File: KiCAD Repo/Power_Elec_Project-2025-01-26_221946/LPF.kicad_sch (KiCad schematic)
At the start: 7 parts, among them U1 LM358

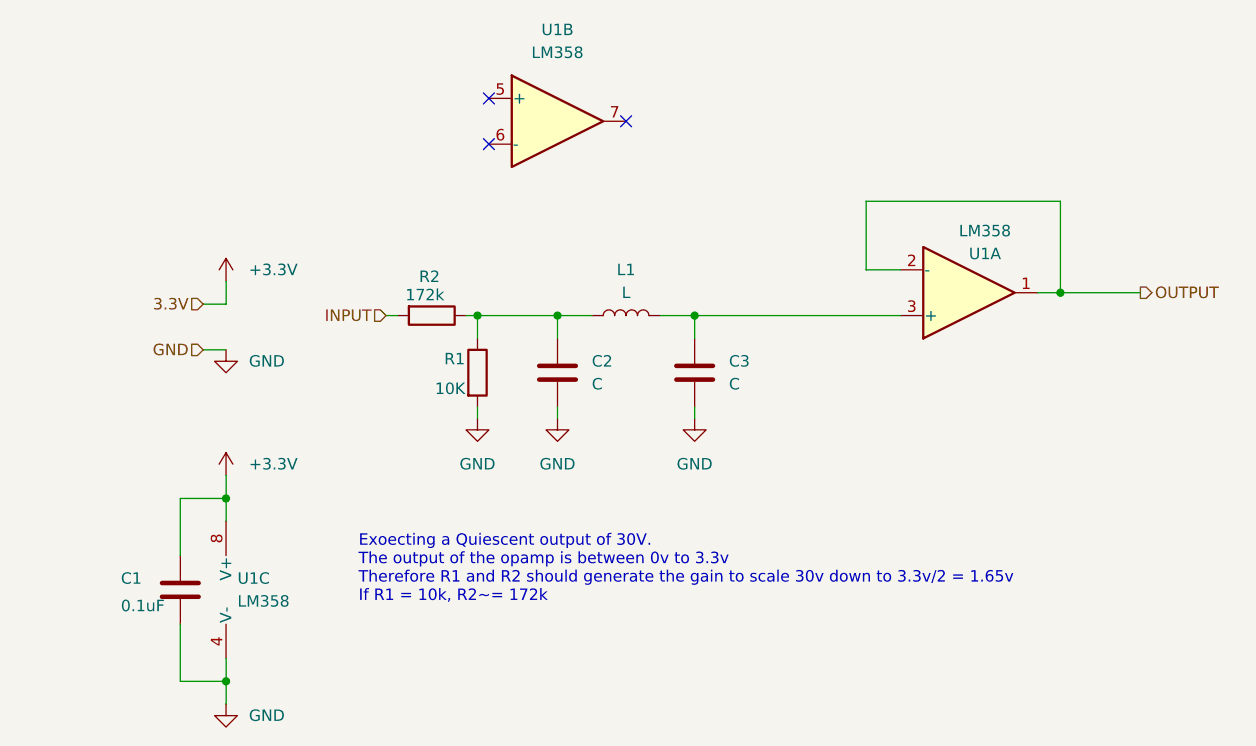
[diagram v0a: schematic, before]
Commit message: lpf design
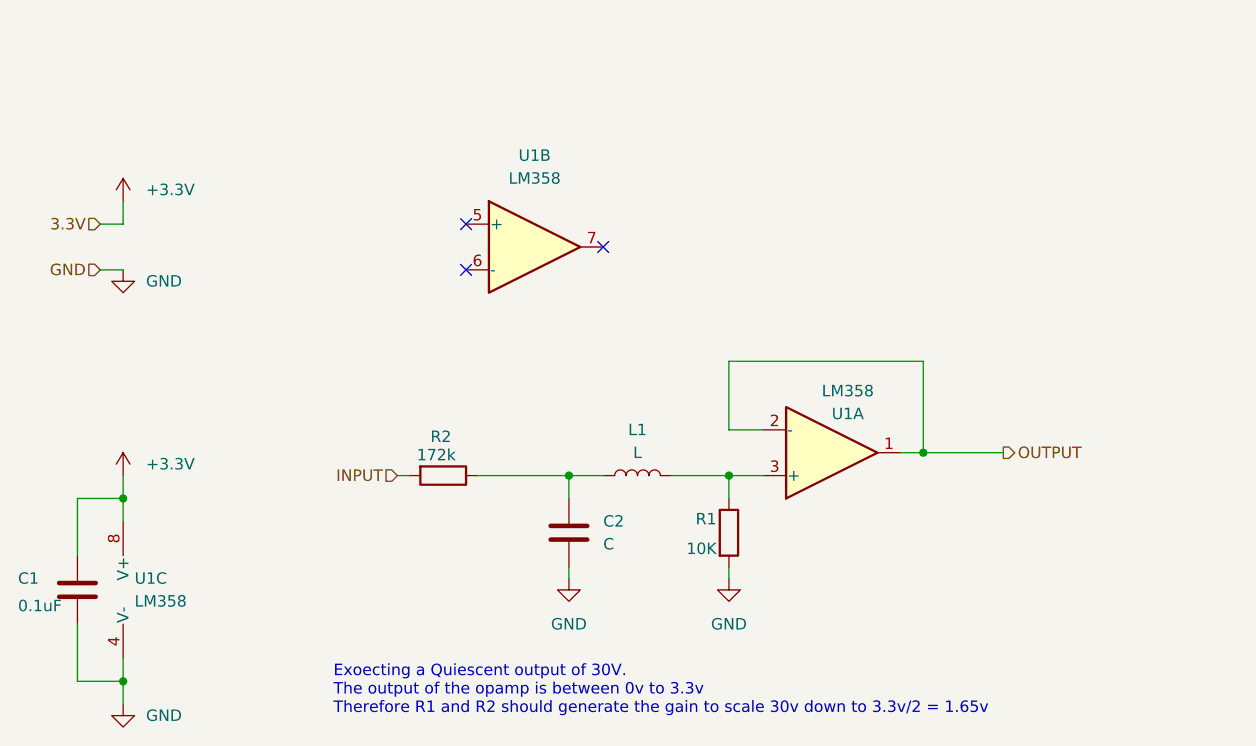
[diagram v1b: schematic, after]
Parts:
- removed C3: C, symbol Device:C
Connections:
- net at L1.2, U1.3 (+): now also R1.1
- net at C2.1, L1.1, R2.1: no longer R1.1
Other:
- note added: "Exoecting a Quiescent output of 30V. The output of the opamp is between 0v to 3.3v Therefore R1 and R2 should generate the gain to scale 30v down to 3.3v/2 = 1.65v"
- note removed: "Exoecting a Quiescent output of 30V. The output of the opamp is between 0v to 3.3v Therefore R1 and R2 should generate the gain to scale 30v down to 3.3v/2 = 1.65v If R1 = 10k, R2~= 172k"
- moved on the sheet: C1, C2, L1, R1, R2, U1A, U1B, U1C
